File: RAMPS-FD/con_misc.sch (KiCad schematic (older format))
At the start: 15 parts, among them K201 SER1, K202 SER2, K203 SER3, K204 SER4, P1 SERIAL1, P2 I2C-1, P211 I2C-0, P213 AUX-4, P214 AUX-2, P215 AUX-3, P216 SERIAL0

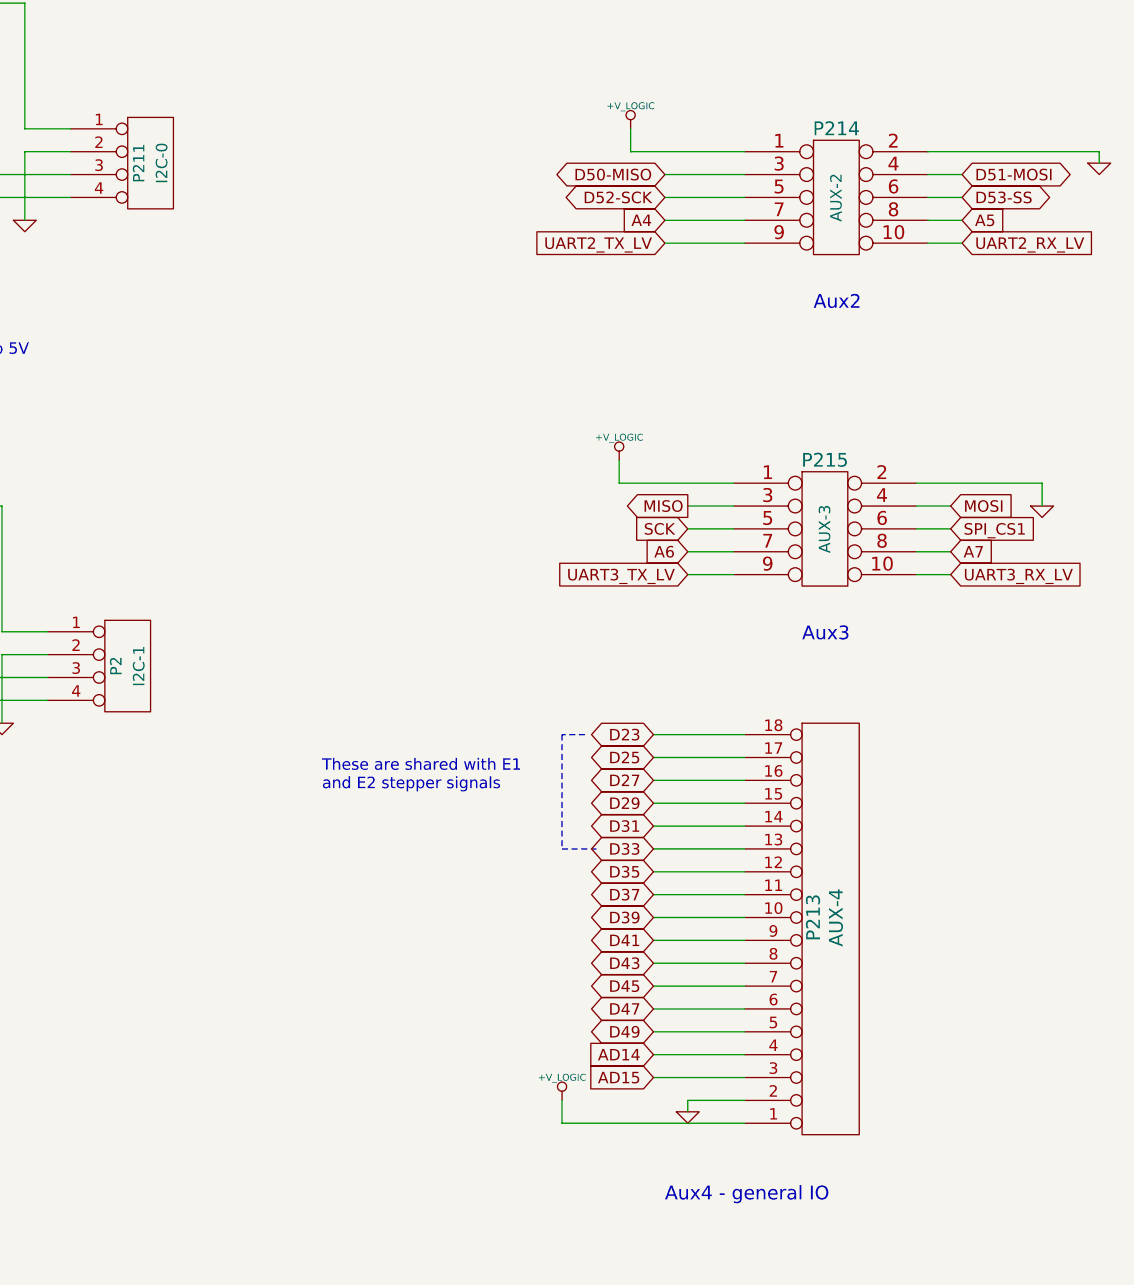
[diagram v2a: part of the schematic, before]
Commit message: RAMPS-FD latest updates
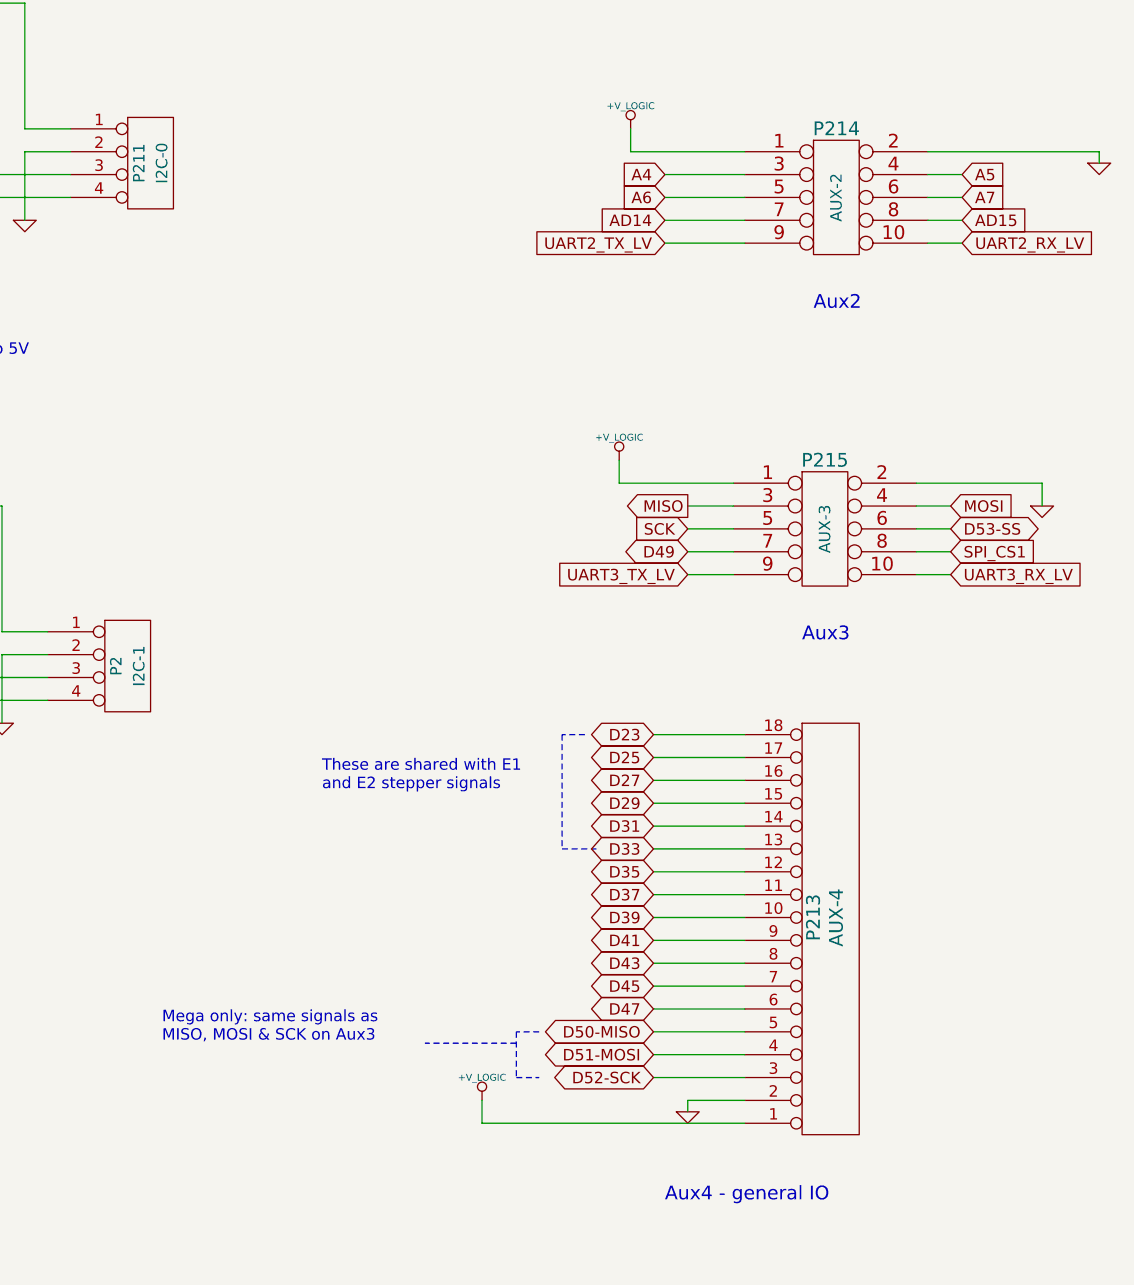
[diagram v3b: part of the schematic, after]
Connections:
- net A4: now also P214.3; no longer P214.7
- net A5: now also P214.4; no longer P214.8
- net A6: now also P214.5; no longer P215.7
- net A7: now also P214.6; no longer P215.8
- net AD14: now also P214.7; no longer P213.4 (P4)
- net AD15: now also P214.8; no longer P213.3 (P3)
- net D49: now also P215.7; no longer P213.5 (P5)
- net D50-MISO: now also P213.5 (P5); no longer P214.3
- net D51-MOSI: now also P213.4 (P4); no longer P214.4
- net D52-SCK: now also P213.3 (P3); no longer P214.5
- net D53-SS: now also P215.6; no longer P214.6
- net SPI_CS1: now also P215.8; no longer P215.6
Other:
- note added: "Mega only: same signals as \nMISO, MOSI & SCK on Aux3"
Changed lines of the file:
@@
 Sheet 6 9
 Title ""
-Date "22 sep 2013"
+Date "23 sep 2013"
 Rev "0.2"
 Comp ""
@@
 Comment4 ""
 $EndDescr
-Text GLabel 8250 6350 0    50   Input ~ 0
+Text GLabel 9600 2600 2    50   Input ~ 0
 AD15
-Text GLabel 8250 6250 0    50   Input ~ 0
+Text GLabel 8300 2600 0    50   Input ~ 0
 AD14
 Wire Wire Line
@@
 	8650 6250 8250 6250
 Wire Wire Line
-	8650 6550 7850 6550
-Wire Wire Line
-	7850 6550 7850 6450
+	8650 6550 7500 6550
+Wire Wire Line
+	7500 6550 7500 6450
 Wire Wire Line
 	9950 3750 9400 3750
@@
 	4950 4450 4950 4600
 Connection ~ 4950 4600
-Text GLabel 8300 2400 0    50   BiDi ~ 0
+Text GLabel 8250 6150 0    50   BiDi ~ 0
 D50-MISO
-Text GLabel 8300 2500 0    50   BiDi ~ 0
+Text GLabel 8250 6350 0    50   BiDi ~ 0
 D52-SCK
 $Comp
@@
 $EndComp
 $Comp
-L GND #PWR067
+L GND #PWR068
 U 1 1 523B601D
 P 5400 4800
-F 0 "#PWR067" H 5400 4800 30  0001 C CNN
+F 0 "#PWR068" H 5400 4800 30  0001 C CNN
 F 1 "GND" H 5400 4730 30  0001 C CNN
 F 2 "" H 5400 4800 60  0001 C CNN
@@
 SCL1
 $Comp
-L +V_LOGIC #PWR068
+L +V_LOGIC #PWR069
 U 1 1 523B601C
 P 4600 3800
-F 0 "#PWR068" H 4600 3770 30  0001 C CNN
+F 0 "#PWR069" H 4600 3770 30  0001 C CNN
 F 1 "+V_LOGIC" H 4600 3900 30  0000 C CNN
 F 2 "" H 4600 3800 60  0001 C CNN
@@
 UART1_TX_LV
 $Comp
-L GND #PWR069
+L GND #PWR070
 U 1 1 523B5AB9
 P 1950 3600
-F 0 "#PWR069" H 1950 3600 30  0001 C CNN
+F 0 "#PWR070" H 1950 3600 30  0001 C CNN
 F 1 "GND" H 1950 3530 30  0001 C CNN
 F 2 "" H 1950 3600 60  0001 C CNN
@@
 Text Notes 550  1950 0    50   ~ 0
 UART-TTL
-Text GLabel 8400 4050 0    50   Input ~ 0
+Text GLabel 8300 2500 0    50   Input ~ 0
 A6
-Text GLabel 9550 4050 2    50   Input ~ 0
+Text GLabel 9600 2500 2    50   Input ~ 0
 A7
-Text GLabel 9600 2600 2    50   Input ~ 0
+Text GLabel 9600 2400 2    50   Input ~ 0
 A5
-Text GLabel 8300 2600 0    50   Input ~ 0
+Text GLabel 8300 2400 0    50   Input ~ 0
 A4
-Text GLabel 9600 2400 2    50   BiDi ~ 0
+Text GLabel 8250 6250 0    50   BiDi ~ 0
 D51-MOSI
 $Comp
-L +V_LOGIC #PWR070
+L +V_LOGIC #PWR071
 U 1 1 517867DE
-P 7850 6450
-F 0 "#PWR070" H 7850 6420 30  0001 C CNN
-F 1 "+V_LOGIC" H 7850 6550 30  0000 C CNN
-F 2 "" H 7850 6450 60  0001 C CNN
-F 3 "" H 7850 6450 60  0001 C CNN
-	1    7850 6450
-	1    0    0    -1
-$EndComp
-$Comp
-L +V_LOGIC #PWR071
+P 7500 6450
+F 0 "#PWR071" H 7500 6420 30  0001 C CNN
+F 1 "+V_LOGIC" H 7500 6550 30  0000 C CNN
+F 2 "" H 7500 6450 60  0001 C CNN
+F 3 "" H 7500 6450 60  0001 C CNN
+	1    7500 6450
+	1    0    0    -1
+$EndComp
+$Comp
+L +V_LOGIC #PWR072
 U 1 1 517867DD
 P 8150 2200
-F 0 "#PWR071" H 8150 2170 30  0001 C CNN
+F 0 "#PWR072" H 8150 2170 30  0001 C CNN
 F 1 "+V_LOGIC" H 8150 2300 30  0000 C CNN
 F 2 "" H 8150 2200 60  0001 C CNN
@@
 $EndComp
 $Comp
-L +V_LOGIC #PWR072
+L +V_LOGIC #PWR073
 U 1 1 517867D0
 P 8100 3650
-F 0 "#PWR072" H 8100 3620 30  0001 C CNN
+F 0 "#PWR073" H 8100 3620 30  0001 C CNN
 F 1 "+V_LOGIC" H 8100 3750 30  0000 C CNN
 F 2 "" H 8100 3650 60  0001 C CNN
@@
 $EndComp
 $Comp
-L +V_LOGIC #PWR073
+L +V_LOGIC #PWR074
 U 1 1 517867C6
 P 4700 1600
-F 0 "#PWR073" H 4700 1570 30  0001 C CNN
+F 0 "#PWR074" H 4700 1570 30  0001 C CNN
 F 1 "+V_LOGIC" H 4700 1700 30  0000 C CNN
 F 2 "" H 4700 1600 60  0001 C CNN
@@
 $EndComp
 $Comp
-L GND #PWR074
+L GND #PWR075
 U 1 1 51084B2C
 P 8400 6500
-F 0 "#PWR074" H 8400 6500 30  0001 C CNN
+F 0 "#PWR075" H 8400 6500 30  0001 C CNN
 F 1 "GND" H 8400 6430 30  0001 C CNN
 F 2 "" H 8400 6500 60  0001 C CNN
@@
 	1    0    0    1
 $EndComp
-Text GLabel 9600 2500 2    50   BiDi ~ 0
+Text GLabel 9550 3950 2    50   BiDi ~ 0
 D53-SS
-Text GLabel 8250 6150 0    50   BiDi ~ 0
+Text GLabel 8400 4050 0    50   BiDi ~ 0
 D49
 Text GLabel 9550 3850 2    50   Input ~ 0
@@
 Must not have external pullups to 5V
 $Comp
-L GND #PWR075
+L GND #PWR076
 U 1 1 5104884C
 P 9950 3850
-F 0 "#PWR075" H 9950 3850 30  0001 C CNN
+F 0 "#PWR076" H 9950 3850 30  0001 C CNN
 F 1 "GND" H 9950 3780 30  0001 C CNN
 F 2 "" H 9950 3850 60  0001 C CNN
@@
 $EndComp
 $Comp
-L GND #PWR076
+L GND #PWR077
 U 1 1 51048839
 P 10200 2350
-F 0 "#PWR076" H 10200 2350 30  0001 C CNN
+F 0 "#PWR077" H 10200 2350 30  0001 C CNN
 F 1 "GND" H 10200 2280 30  0001 C CNN
 F 2 "" H 10200 2350 60  0001 C CNN
@@
 $EndComp
 $Comp
-L GND #PWR077
+L GND #PWR078
 U 1 1 5104861F
 P 1950 2350
-F 0 "#PWR077" H 1950 2350 30  0001 C CNN
+F 0 "#PWR078" H 1950 2350 30  0001 C CNN
 F 1 "GND" H 1950 2280 30  0001 C CNN
 F 2 "" H 1950 2350 60  0001 C CNN
@@
 $EndComp
 $Comp
-L GND #PWR078
+L GND #PWR079
 U 1 1 51047C7E
 P 1550 6850
-F 0 "#PWR078" H 1550 6850 30  0001 C CNN
+F 0 "#PWR079" H 1550 6850 30  0001 C CNN
 F 1 "GND" H 1550 6780 30  0001 C CNN
 F 2 "" H 1550 6850 60  0001 C CNN
@@
 $EndComp
 $Comp
-L +5V #PWR079
+L +5V #PWR080
 U 1 1 51047C7D
 P 1550 6450
-F 0 "#PWR079" H 1550 6540 20  0001 C CNN
+F 0 "#PWR080" H 1550 6540 20  0001 C CNN
 F 1 "+5V" H 1550 6540 30  0000 C CNN
 F 2 "" H 1550 6450 60  0001 C CNN
@@
 SERVO3
 $Comp
-L +5V #PWR080
+L +5V #PWR081
 U 1 1 51047C7B
 P 1550 5700
-F 0 "#PWR080" H 1550 5790 20  0001 C CNN
+F 0 "#PWR081" H 1550 5790 20  0001 C CNN
 F 1 "+5V" H 1550 5790 30  0000 C CNN
 F 2 "" H 1550 5700 60  0001 C CNN
@@
 $EndComp
 $Comp
-L GND #PWR081
+L GND #PWR082
 U 1 1 51047C7A
 P 1550 6100
-F 0 "#PWR081" H 1550 6100 30  0001 C CNN
+F 0 "#PWR082" H 1550 6100 30  0001 C CNN
 F 1 "GND" H 1550 6030 30  0001 C CNN
 F 2 "" H 1550 6100 60  0001 C CNN
@@
 $EndComp
 $Comp
-L GND #PWR082
+L GND #PWR083
 U 1 1 51047C77
 P 1550 5450
-F 0 "#PWR082" H 1550 5450 30  0001 C CNN
+F 0 "#PWR083" H 1550 5450 30  0001 C CNN
 F 1 "GND" H 1550 5380 30  0001 C CNN
 F 2 "" H 1550 5450 60  0001 C CNN
@@
 $EndComp
 $Comp
-L +5V #PWR083
+L +5V #PWR084
 U 1 1 51047C76
 P 1550 5050
-F 0 "#PWR083" H 1550 5140 20  0001 C CNN
+F 0 "#PWR084" H 1550 5140 20  0001 C CNN
 F 1 "+5V" H 1550 5140 30  0000 C CNN
 F 2 "" H 1550 5050 60  0001 C CNN
@@
 SERVO1
 $Comp
-L +5V #PWR084
+L +5V #PWR085
 U 1 1 51047C09
 P 1550 4300
-F 0 "#PWR084" H 1550 4390 20  0001 C CNN
+F 0 "#PWR085" H 1550 4390 20  0001 C CNN
 F 1 "+5V" H 1550 4390 30  0000 C CNN
 F 2 "" H 1550 4300 60  0001 C CNN
@@
 $EndComp
 $Comp
-L GND #PWR085
+L GND #PWR086
 U 1 1 51047C01
 P 1550 4700
-F 0 "#PWR085" H 1550 4700 30  0001 C CNN
+F 0 "#PWR086" H 1550 4700 30  0001 C CNN
 F 1 "GND" H 1550 4630 30  0001 C CNN
 F 2 "" H 1550 4700 60  0001 C CNN
@@
 SDA
 $Comp
-L GND #PWR086
+L GND #PWR087
 U 1 1 51047413
 P 5500 2600
-F 0 "#PWR086" H 5500 2600 30  0001 C CNN
+F 0 "#PWR087" H 5500 2600 30  0001 C CNN
 F 1 "GND" H 5500 2530 30  0001 C CNN
 F 2 "" H 5500 2600 60  0001 C CNN
@@
 Text Notes 550  1600 0    50   ~ 0
 Note: this serial port is shared with\nUSB programming port
-Text GLabel 9550 3950 2    50   Input ~ 0
+Text GLabel 9550 4050 2    50   Input ~ 0
 SPI_CS1
 Wire Wire Line
@@
 Text Notes 6800 5100 0    50   ~ 0
 These are shared with E1 \nand E2 stepper signals
+Wire Notes Line
+	7750 6150 7650 6150
+Wire Notes Line
+	7650 6150 7650 6350
+Wire Notes Line
+	7650 6350 7750 6350
+Wire Notes Line
+	7650 6200 7250 6200
+Text Notes 6100 6200 0    50   ~ 0
+Mega only: same signals as \nMISO, MOSI & SCK on Aux3
 $EndSCHEMATC
